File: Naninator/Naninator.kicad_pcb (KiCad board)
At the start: 2 copper layers, 43.2 x 17.8 mm, 27 parts, among them J1 CONN_02X03, J101 USB_OTG, J2 CONN_01X15, J3 CONN_01X15, U001 FT232RL, U201 MAX8881, U401 ATMEGA328P-M, Y406 16MHz

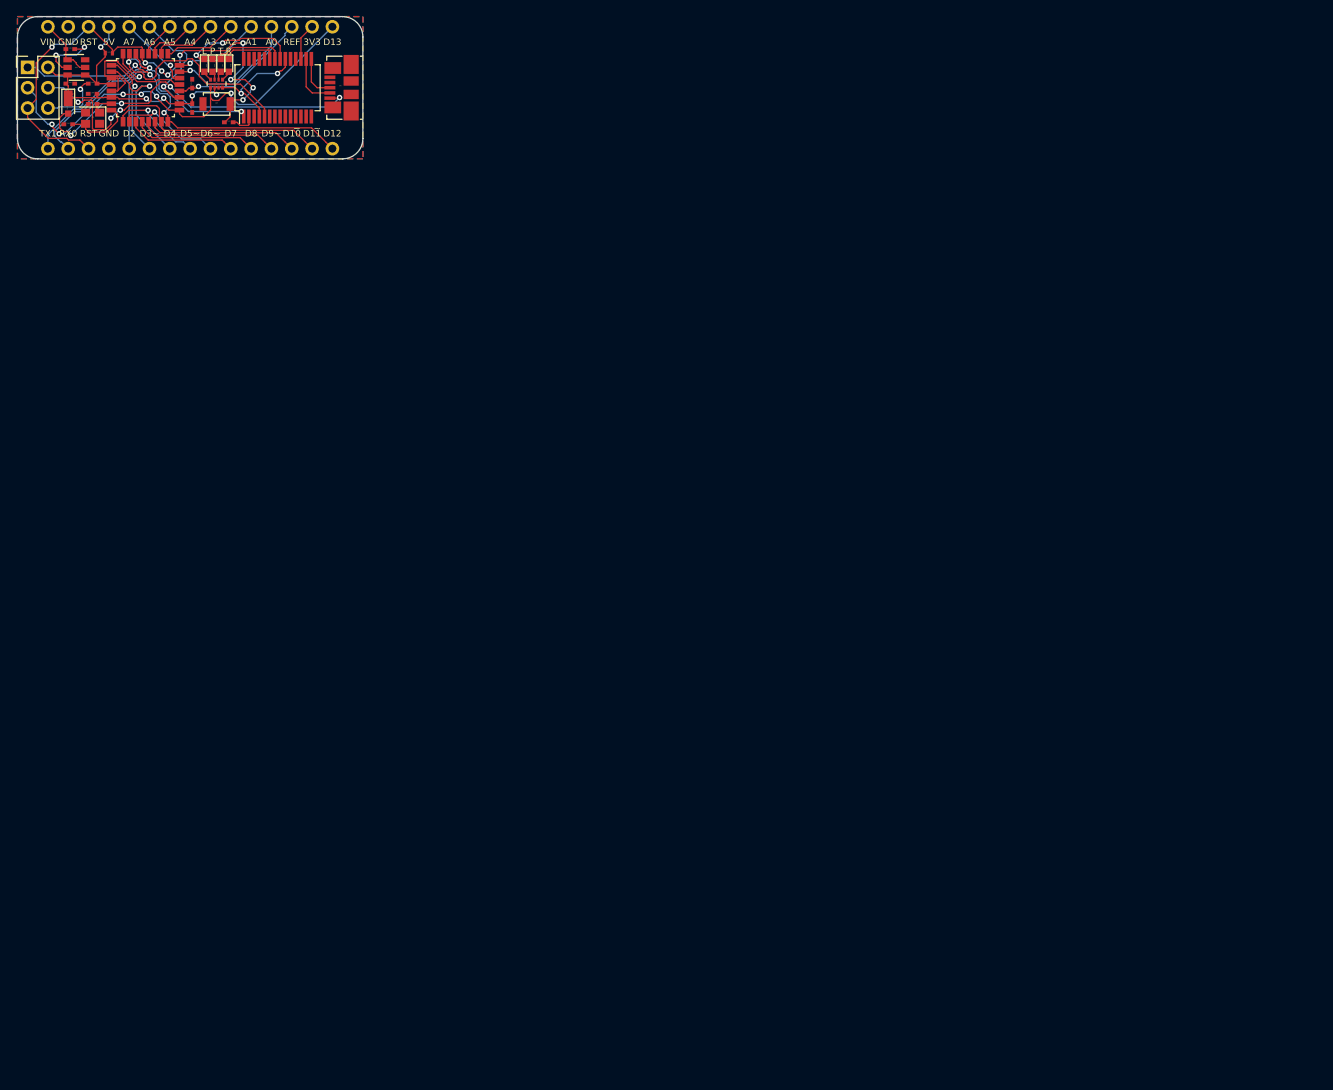
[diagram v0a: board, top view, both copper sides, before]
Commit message: Consistentized the Naninator, Tomo, and Tomo Plugin
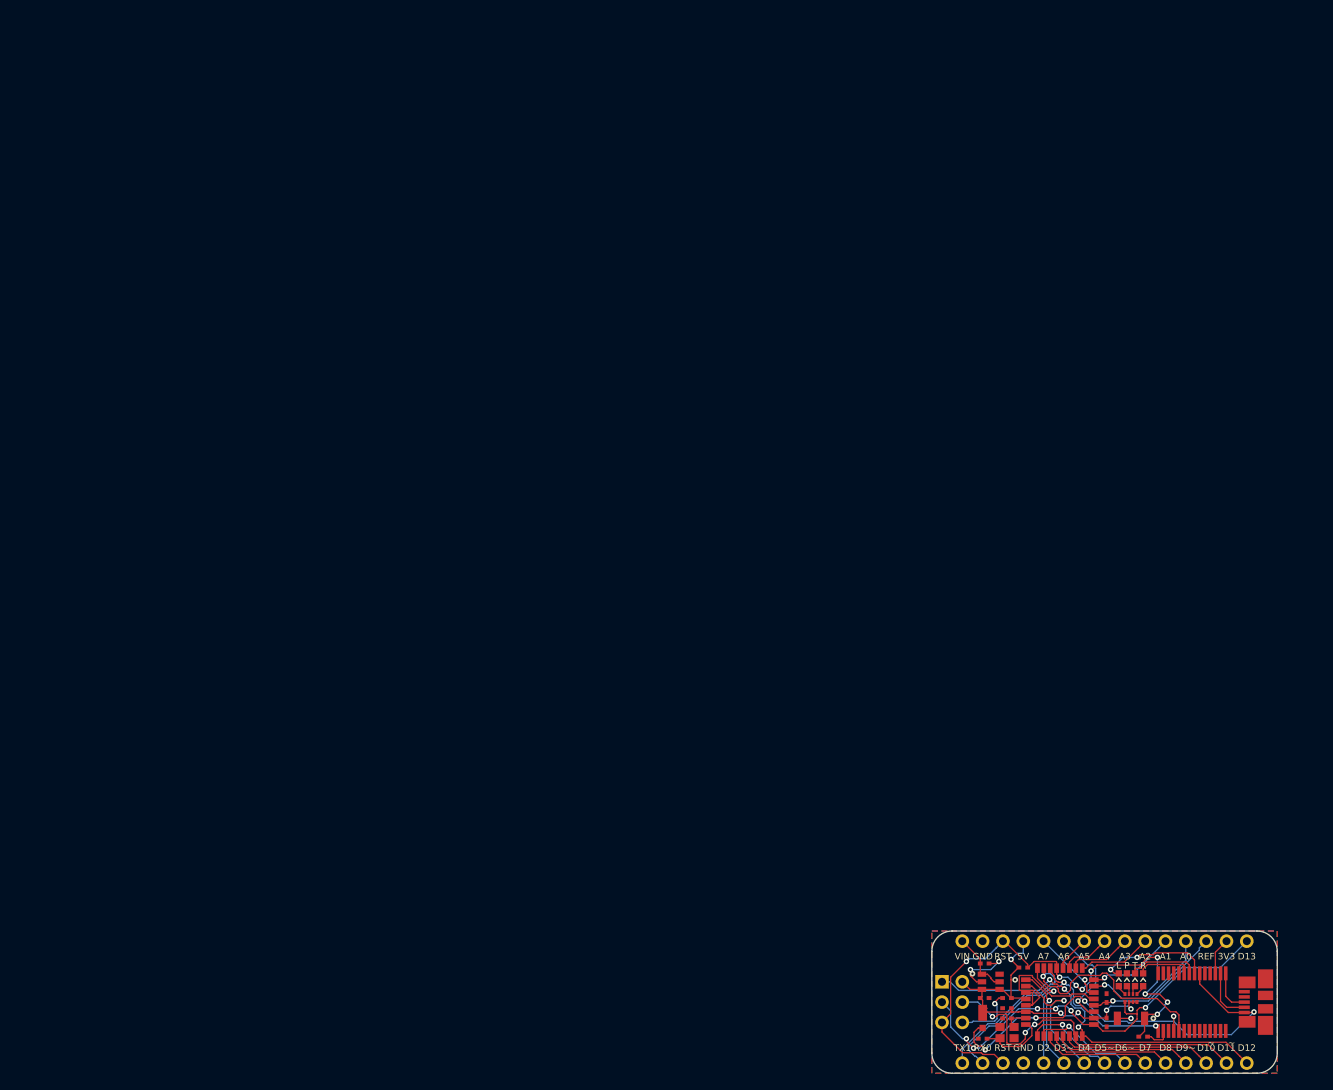
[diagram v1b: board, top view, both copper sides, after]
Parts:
- added REF**: KiCAD Logo, KwanSystems:Symbol_KiCAD-Logo_CopperAndSilkScreenTop_small, B.Cu at (122.7, 110.2)
- C404, C406, C418, C420: footprint Capacitors_SMD:C_0402_NoSilk -> KwanSystems:SMD_0402
- C407, C408: value 18pF -> 22pF; footprint Capacitors_SMD:C_0402_NoSilk -> KwanSystems:SMD_0402
- D003: value D_Schottky -> MSSP12L
- D022: renamed from D22; footprint LEDs:LED_0603 -> KwanSystems:D_0603
- D023: renamed from D203; footprint LEDs:LED_0603 -> KwanSystems:D_0603
- D401, D402: footprint LEDs:LED_0603 -> KwanSystems:D_0603
- G***: footprint KwanSystems:KWAN_CIRCLE -> KwanSystems:KWAN_CIRCLE_soldermask
- J101: value USB_OTG -> USB_MICROB
- R429: footprint Resistors_SMD:R_0402_NoSilk -> KwanSystems:SMD_0402
- S429: footprint Buttons_Switches_SMD:SW_SPST_B3U-1000P -> KwanSystems:SW_SPST_B3U-1000P
- U201: value MAX8881 -> MAX8881 5V
- U401: value ATMEGA328P-M -> ATMEGA328P-AU
- moved C102 161.6 mm to (140.7, 109.7)
- moved C201 161.6 mm to (120.9, 100.6)
- moved C203 161.6 mm to (120.9, 104.9)
- moved C404 161.6 mm to (123.7, 104.9)
- moved C406 161.6 mm to (123.7, 106.2)
- moved C407 161.6 mm to (123.7, 107.4), turned to 0 degrees
- moved C408 161.6 mm to (120.7, 110.0)
- moved C418 161.6 mm to (136.1, 108.0)
- moved C420 161.6 mm to (136.1, 104.9)
- moved D003 161.6 mm to (120.7, 107.7)
- moved D023 161.6 mm to (140.7, 102.6)
- moved D401 161.6 mm to (138.7, 102.6)
- moved D402 161.6 mm to (137.7, 102.6)
- moved J1 161.6 mm to (115.6, 102.9)
- moved J101 161.6 mm to (154.7, 105.4)
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- renumbered Y406 to Y407
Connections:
- net /D0 renamed /D0/RX
- net /D1 renamed /D1/TX
- net /XTAL2 renamed /ATmega/XTAL2
- C203 pad 1: VCC -> +5V
- C404 pad 1: VCC -> +5V
- C406 pad 1: VCC -> +5V
- C407 pad 1: /XTAL1 -> GND
- C407 pad 2: GND -> /ATmega/XTAL1
- C418 pad 1: VCC -> +5V
- D003 pad 1: VCC -> +5V
- J1 pad 2: VCC -> +5V
- J101 pad 4: GND -> (no net)
- J3 pad 12: VCC -> +5V
- R1 pad 6: VCC -> +5V
- R1 pad 7: VCC -> +5V
- R1 pad 8: VCC -> +5V
- R429 pad 1: VCC -> +5V
- U001 pad 10: Net-(U001-Pad10) -> (no net)
- U001 pad 11: Net-(U001-Pad11) -> (no net)
- U001 pad 12: Net-(U001-Pad12) -> (no net)
- U001 pad 13: Net-(U001-Pad13) -> (no net)
- U001 pad 14: Net-(U001-Pad14) -> (no net)
- U001 pad 19: Net-(U001-Pad19) -> (no net)
- U001 pad 20: VCC -> /VBUS
- U001 pad 27: Net-(U001-Pad27) -> (no net)
- U001 pad 28: Net-(U001-Pad28) -> (no net)
- U001 pad 3: Net-(U001-Pad3) -> (no net)
- U001 pad 4: VCC -> /VBUS
- U001 pad 6: Net-(U001-Pad6) -> (no net)
- U001 pad 9: Net-(U001-Pad9) -> (no net)
- U201 pad 3: VCC -> +5V
- U201 pad 4: VCC -> +5V
- U201 pad 6: Net-(U201-Pad6) -> (no net)
- U401 pad 18: VCC -> +5V
- U401 pad 4: VCC -> +5V
- U401 pad 6: VCC -> +5V
- U401 pad 7: /XTAL1 -> /ATmega/XTAL1
- Y407 pad 1: /XTAL1 -> /ATmega/XTAL1
- Y407 pad 4: Net-(Y406-Pad4) -> GND
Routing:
- net VCC: track 59.1 -> 0.00 mm, vias 7 -> 0
- net +5V: track 0.00 -> 45.0 mm, vias 0 -> 5
- net /VBUS: track 44.5 -> 56.8 mm, vias 4 -> 5
- net /XTAL1: track 3.03 -> 0.00 mm
- net /ATmega/XTAL1: track 0.00 -> 3.03 mm
- net GND: track 50.5 -> 52.2 mm, vias 5 -> 6
- net /A6: track 13.9 -> 13.0 mm
- net /D1/TX: track 44.7 -> 45.3 mm
- net /D13: track 54.2 -> 53.6 mm
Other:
- board text added: "01 Aug 2017"
- board text added: "Designed with"
- board text added: "github.com/kwan3217"
- board text removed: "01 Apr 2017"
- board text removed: "stkwans.blogspot.com"

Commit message: Rework to solve solder mask problem and use 1206 parts
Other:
- rule pad_to_mask_clearance: 0.2 -> 0
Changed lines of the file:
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@@
-(kicad_pcb (version 4) (host pcbnew 4.0.5+dfsg1-4)
+(kicad_pcb (version 20170123) (host pcbnew no-vcs-found-f042fcd~59~ubuntu17.04.1)
   (general
-    (links 102)
-    (no_connects 1)
-    (area 114.224999 96.444999 157.555001 114.375001)
     (thickness 1.6)
     (drawings 56)
@@
     (pad_size 0.5 0.381)
     (pad_drill 0)
-    (pad_to_mask_clearance 0.2)
+    (pad_to_mask_clearance 0)
     (aux_axis_origin 114.3 114.3)
     (grid_origin 114.3 114.3)
@@
       (hpglpenspeed 20)
       (hpglpendiameter 15)
-      (hpglpenoverlay 2)
       (psnegative false)
       (psa4output false)
@@
     (pad 6 smd rect (at -1.33 0.84 180) (size 1.9 1.175) (layers F.Cu F.Paste F.Mask)
       (net 3 GND))
-    (model Connectors_Molex.3dshapes/USB_Micro-B_Molex_47346-0001.wrl
-      (at (xyz -0.05 0 0.05))
-      (scale (xyz 0.39 0.39 0.39))
+    (model /home/chrisj/workspace/kicad/KwanSystems.pretty/wrl/Molex_47346_0001.wrl
+      (at (xyz -0.03937007874015748 0 0))
+      (scale (xyz 0.3937 0.3937 0.3937))
       (rotate (xyz -90 0 90))
     )
@@
     (tags "resistor array")
     (attr smd)
-    (fp_text reference R1 (at -0.127 0 360) (layer F.SilkS) hide
+    (fp_text reference R1 (at -0.127 0) (layer F.SilkS) hide
       (effects (font (size 0.127 0.127) (thickness 0.01524)))
     )
-    (fp_text value 680 (at 0.127 0 360) (layer F.Fab)
+    (fp_text value 680 (at 0.127 0) (layer F.Fab)
       (effects (font (size 0.1016 0.1016) (thickness 0.01524)))
     )
@@
     (pad 2 smd rect (at 1.7 0 180) (size 0.9 1.7) (layers F.Cu F.Paste F.Mask)
       (net 3 GND))
-    (model ../KwanSystems.pretty/B3U1000P.wrl
+    (model /home/chrisj/workspace/kicad/KwanSystems.pretty/wrl/B3U1000P.wrl
       (at (xyz 0 0 0))
       (scale (xyz 0.3937 0.3937 0.3937))
@@
     (model Diodes_SMD.3dshapes/D_TUMD2.wrl
       (at (xyz 0 0 0))
-      (scale (xyz 4 4 4))
-      (rotate (xyz 0 0 180))
+      (scale (xyz 1 1 1))
+      (rotate (xyz 0 0 0))
     )
   )
@@
       (net 6 /D12))
     (model Pin_Headers.3dshapes/Pin_Header_Straight_1x15_Pitch2.54mm.wrl
-      (at (xyz 0 -0.7 0))
-      (scale (xyz 1 1 1))
-      (rotate (xyz 0 0 90))
+      (at (xyz 0 0 0))
+      (scale (xyz 1 1 1))
+      (rotate (xyz 0 0 0))
     )
   )
@@
       (net 3 GND))
     (model Pin_Headers.3dshapes/Pin_Header_Straight_2x03_Pitch2.54mm.wrl
-      (at (xyz 0.05 -0.1 0))
-      (scale (xyz 1 1 1))
-      (rotate (xyz 0 0 90))
+      (at (xyz 0 0 0))
+      (scale (xyz 1 1 1))
+      (rotate (xyz 0 0 0))
     )
   )
@@
       (net 2 HT))
     (model Pin_Headers.3dshapes/Pin_Header_Straight_1x15_Pitch2.54mm.wrl
-      (at (xyz 0 -0.7 0))
-      (scale (xyz 1 1 1))
-      (rotate (xyz 0 0 90))
+      (at (xyz 0 0 0))
+      (scale (xyz 1 1 1))
+      (rotate (xyz 0 0 0))
     )
   )
@@
     (pad 1 smd rect (at -0.55 0) (size 0.6 0.5) (layers F.Cu F.Paste F.Mask)
       (net 36 +5V))
-    (model Capacitors_SMD.3dshapes/C_0402.wrl
-      (at (xyz 0 0 0))
-      (scale (xyz 1 1 1))
+    (model ${KISYS3DMOD}/Resistors_SMD.3dshapes/R_0402.wrl
+      (at (xyz 0 0 0))
+      (scale (xyz 1 1 1))

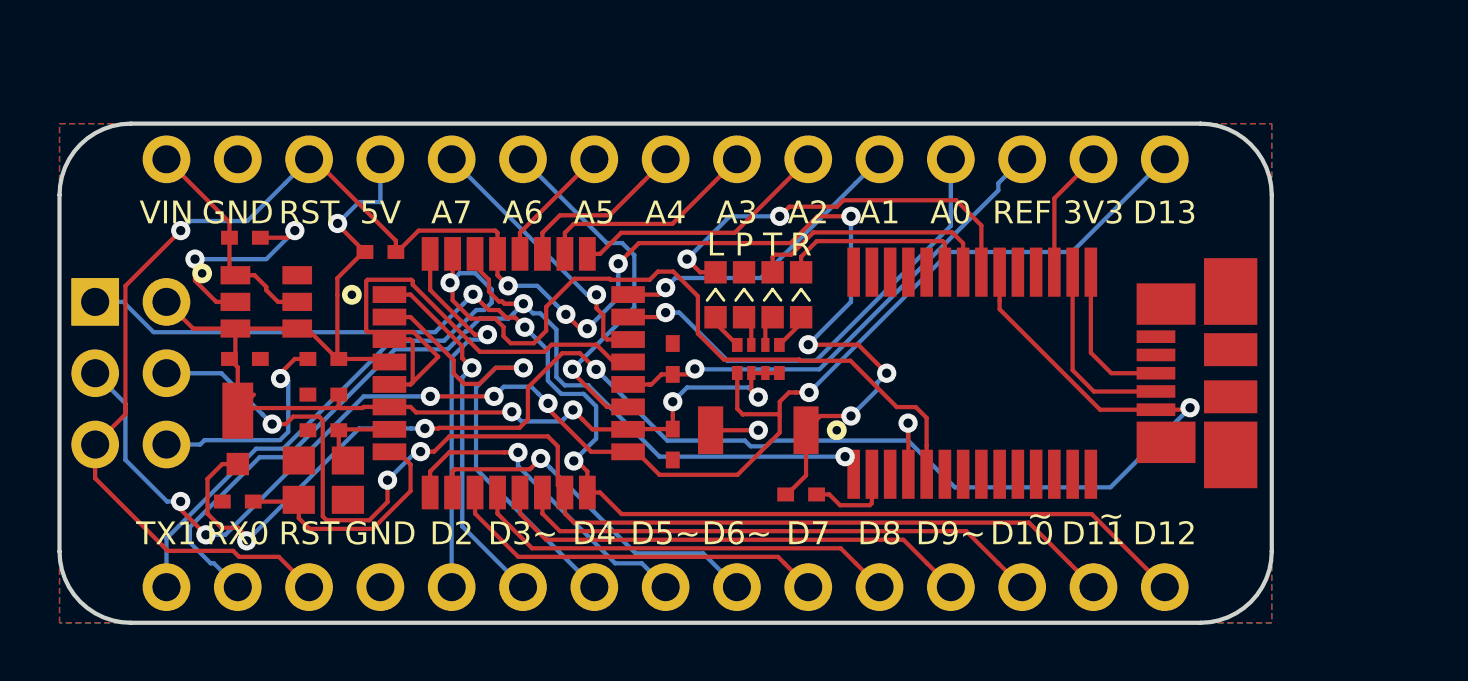
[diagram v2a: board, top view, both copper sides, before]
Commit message: j
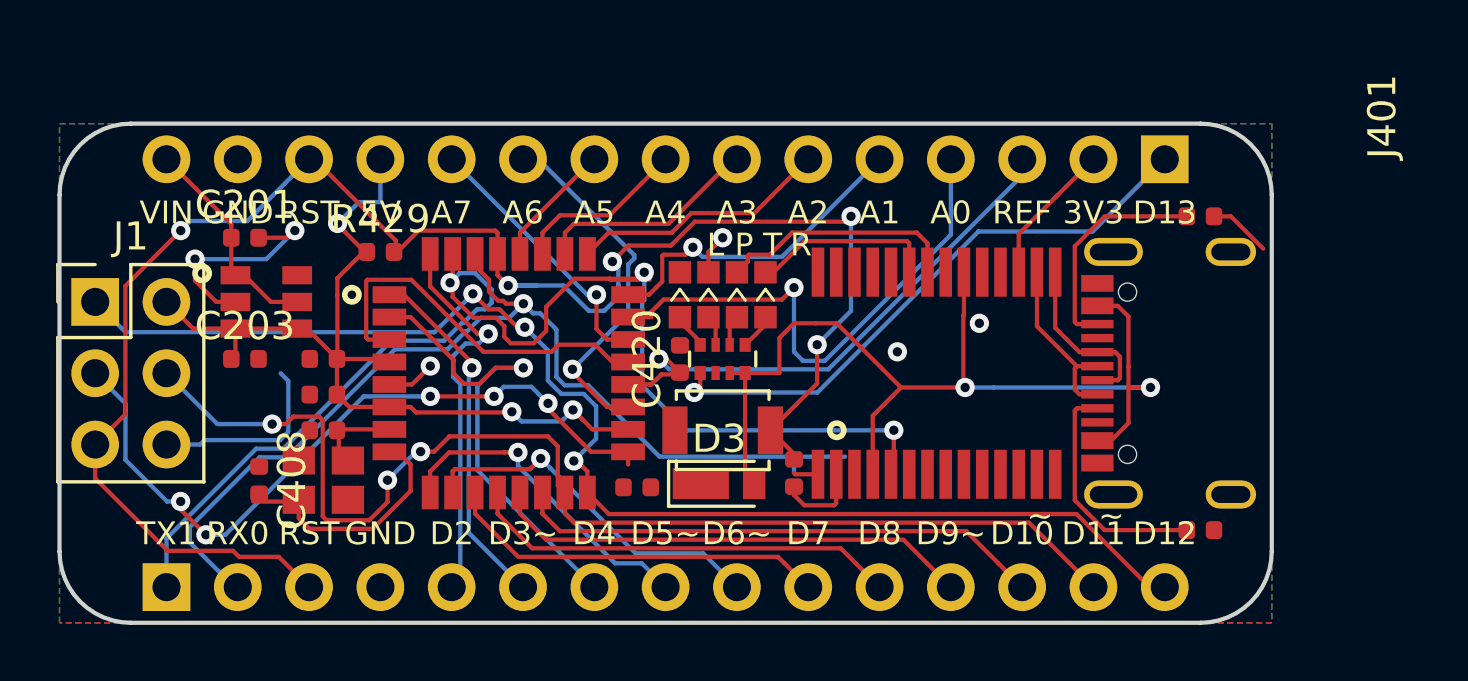
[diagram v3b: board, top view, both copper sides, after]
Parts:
- removed G***: LOGO, KwanSystems:KWAN_CIRCLE_soldermask
- removed J101: USB_MICROB, Connectors_Molex:USB_Micro-B_Molex_47346-0001
- removed REF**: KiCAD Logo, KwanSystems:Symbol_KiCAD-Logo_CopperAndSilkScreenTop_small
- removed REF***: OSHW-Symbol_6.7x6mm_SilkScreen, Symbols:OSHW-Symbol_6.7x6mm_SilkScreen
- added G101: Designed With, KwanSystems:Symbol_KiCAD-Logo_CopperAndSilkScreenTop_small, B.Cu at (145.3, 106.2)
- added G102: KwanSystems, KwanSystems:StKwansSoldermask, B.Cu at (152.4, 105.4)
- added J401: USB_C_Receptacle_USB2.0, KwanSystems:GCTUSBTypeC_PTH, F.Cu at (158.6, 105.4)
- added R401: 5.1k, Resistor_SMD:R_0402_1005Metric, F.Cu at (154.9, 111.0)
- added R402: 5.1k, Resistor_SMD:R_0402_1005Metric, F.Cu at (154.9, 99.8)
- C201, C203: footprint Capacitors_SMD:C_0402_NoSilk -> Capacitor_SMD:C_0402_1005Metric
- C302: renamed from C102; footprint Capacitors_SMD:C_0402_NoSilk -> Capacitor_SMD:C_0402_1005Metric
- C404, C406, C407, C408, C418, C420: footprint KwanSystems:SMD_0402 -> Capacitor_SMD:C_0402_1005Metric
- D3: renamed from D003; footprint KwanSystems:MicroSMP -> Diode_SMD:D_TUMD2
- J1: footprint Pin_Headers:Pin_Header_Straight_2x03_Pitch2.54mm -> Connector_PinHeader_2.54mm:PinHeader_2x03_P2.54mm_Vertical
- J2, J3: footprint Pin_Headers:Pin_Header_Straight_1x15_Pitch2.54mm -> Connector_PinHeader_2.54mm:PinHeader_1x15_P2.54mm_Vertical
- R201: renamed from R1; footprint Resistors_SMD:R_Array_Convex_4x0402 -> KwanSystems:R_Array_Convex_4x0402
- R429: footprint KwanSystems:SMD_0402 -> Resistor_SMD:R_0402_1005Metric
- moved D3 17.2 mm to (137.8, 109.3), turned to 0 degrees
- moved C418 1.98 mm to (134.9, 109.5), turned to 180 degrees
- moved D323 1.27 mm to (139.4, 102.6)
- moved D401 1.27 mm to (137.4, 102.6)
- moved D402 1.27 mm to (136.4, 102.6)
- moved R201 1.27 mm to (137.9, 104.9)
- moved S429 1.27 mm to (137.9, 107.4)
- moved U301 1.27 mm to (145.5, 105.4)
- moved D322 1.27 mm to (138.4, 102.6)
- moved C408 1.08 mm to (121.4, 109.2), turned to 270 degrees
- moved C302 0.80 mm to (140.5, 109.0), turned to 90 degrees
- moved C420 0.25 mm to (136.4, 104.9)
- renumbered D022 to D322, D023 to D323, U001 to U301
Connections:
- net /DTR renamed /USB Serial/DTR
- net /RESET renamed /~RESET
- net /RX_LED+ renamed /USB Serial/RX_LED+
- net /RX_LED- renamed /USB Serial/RX_LED-
- net /TX_LED+ renamed /USB Serial/TX_LED+
- net /TX_LED- renamed /USB Serial/TX_LED-
- C203 pad 1: +5V -> VCC
- C404 pad 1: +5V -> VCC
- C406 pad 1: +5V -> VCC
- C418 pad 1: +5V -> VCC
- D3 pad 1: +5V -> VCC
- J1 pad 2: +5V -> VCC
- J3 pad 12: +5V -> VCC
- R201 pad 6: +5V -> VCC
- R201 pad 7: +5V -> /VBUS
- R201 pad 8: +5V -> /VBUS
- R429 pad 1: +5V -> VCC
- U201 pad 3: +5V -> VCC
- U201 pad 4: +5V -> VCC
- U301 pad 15: /D+ -> /USB Serial/D+
- U301 pad 16: /D- -> /USB Serial/D-
- U401 pad 18: +5V -> VCC
- U401 pad 4: +5V -> VCC
- U401 pad 6: +5V -> VCC
- Y407 pad 4: GND -> (no net)
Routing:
- net +5V: track 45.0 -> 0.00 mm, vias 5 -> 0
- net VCC: track 0.00 -> 31.6 mm, vias 0 -> 3
- net /VBUS: track 56.8 -> 37.5 mm, vias 5 -> 2
- net GND: track 52.2 -> 34.1 mm
- net /USB Serial/USB-C Connector/CC1: track 0.00 -> 8.46 mm
- net /USB Serial/USB-C Connector/CC2: track 0.00 -> 7.96 mm
- net /D-: track 6.77 -> 0.00 mm
- net /USB Serial/D-: track 0.00 -> 6.40 mm
- net /USB Serial/D+: track 0.00 -> 6.31 mm
- net /D13: track 53.6 -> 47.7 mm
- net /D+: track 5.49 -> 0.00 mm
- net /~RESET: track 65.9 -> 63.1 mm, vias 9 -> 5
- net /A0: track 16.6 -> 19.0 mm
- net /AREF: track 17.6 -> 19.3 mm
- net /D1/TX: track 45.3 -> 47.0 mm, vias 1 -> 3
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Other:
- rule via_min_size: 0.6858 -> 0.508
- board text added: "10 Sep 2020"
- board text added: "Naninator 1.2"
- board text removed: "01 Aug 2017"
- board text removed: "Designed with"
- board text removed: "Naninator 1.1"
- board text removed: "St Kwan's Home for"
- board text removed: "a division of Kwan Systems"
- board text removed: "github.com/kwan3217"
- board text removed: "the Terminally ADD"
